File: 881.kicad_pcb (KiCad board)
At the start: 2 copper layers, 38 x 105 mm, 79 parts, among them J1 BD TRIG, J10 CY TRIG, J11 OH TRIG, J12 CH_TRIG, J13 ACCENT IN, J14 RUN/STOP, J15 RESET, J16 CLOCK OUT, J17 ACCENT OUT, J2 SD TRIG, J3 LT TRIG, J4 MT TRIG, J5 HT_TRIG, J6 RS TRIG, J7 CP_TRIG, J8 MA_TRIG, J9 CB TRIG, P1 CONN_02X03, P2 CONN_02X10, SW1 SPDT, U1 CD4048B, U2 CD4048B, X1 SYNC24 OUT, X2 MIDI OUT

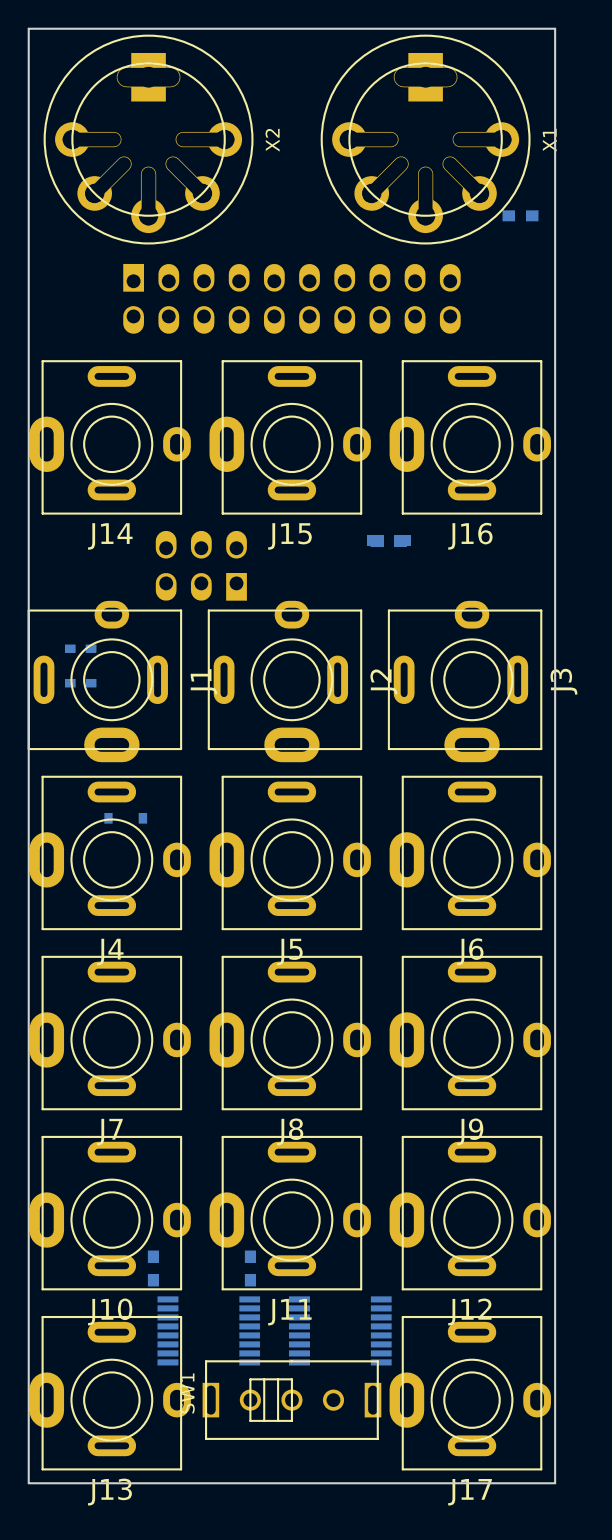
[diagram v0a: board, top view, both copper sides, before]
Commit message: placed and routed
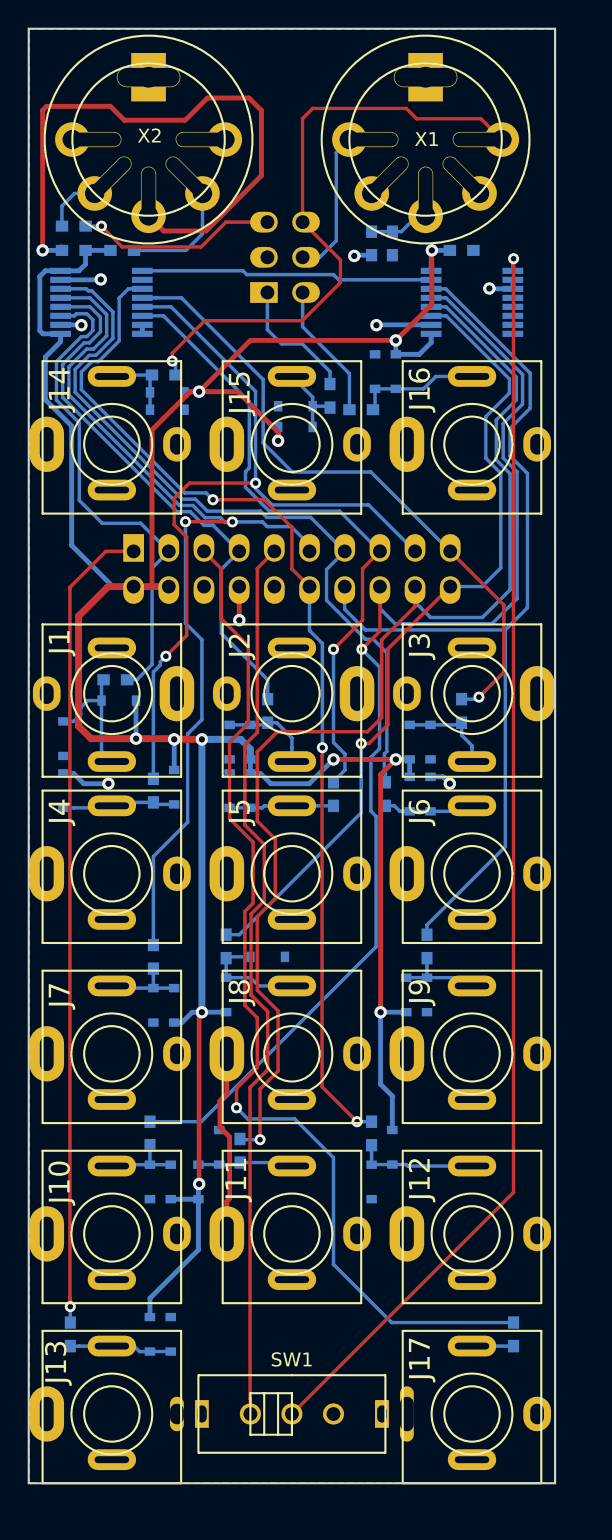
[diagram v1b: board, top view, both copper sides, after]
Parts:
- SW1: footprint MyModules:SS-12F45-1P2T-SLIDE -> MyModules:SS-12F108-1P2T-SLIDE
- moved C3 75.1 mm to (142.8, 71.0), turned to 0 degrees
- moved U2 74.9 mm to (143.5, 74.8)
- moved U1 74.7 mm to (116.8, 74.8)
- moved C2 73.7 mm to (114.8, 71.0), turned to 180 degrees
- moved R16 61.7 mm to (114.5, 149.2), turned to 90 degrees
- moved D25 59.8 mm to (120.2, 149.2), turned to 90 degrees
- moved D26 59.4 mm to (121.8, 149.2), turned to 270 degrees
- moved R20 58.0 mm to (146.5, 149.2), turned to 90 degrees
- moved D20 49.4 mm to (120.2, 138.2), turned to 90 degrees
- moved D19 48.9 mm to (121.8, 138.2), turned to 270 degrees
- moved D21 48.3 mm to (123.8, 138.2), turned to 270 degrees
- moved D24 46.3 mm to (136.2, 138.2), turned to 90 degrees
- moved R12 46.1 mm to (120.2, 134.8), turned to 90 degrees
- moved D22 45.5 mm to (125.2, 135.8), turned to 270 degrees
- moved R13 45.3 mm to (126.8, 136.0), turned to 90 degrees
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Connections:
- U1 pad 11: /RS_TRIG -> /BD_TRIG
- U1 pad 12: /CP_TRIG -> /SD_TRIG
- U1 pad 13: /SD_TRIG -> /CP_TRIG
- U1 pad 14: /BD_TRIG -> /RS_TRIG
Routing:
- net +5V: track 0.00 -> 218.0 mm, vias 0 -> 12
- net Net-(SW1-Pad2): track 0.00 -> 90.9 mm, vias 0 -> 1
- net /CY_TRIG: track 0.00 -> 87.8 mm, vias 0 -> 1
- net /OH_TRIG: track 0.00 -> 86.1 mm, vias 0 -> 1
- net GND: track 0.00 -> 76.8 mm, vias 0 -> 9
- net COMMON_TRIG: track 0.00 -> 75.4 mm, vias 0 -> 1
- net /CH_TRIG: track 0.00 -> 75.2 mm, vias 0 -> 3
- net /CP_TRIG: track 0.00 -> 69.3 mm, vias 0 -> 2
- net /CB_TRIG: track 0.00 -> 68.2 mm
- net /TRIG: track 0.00 -> 65.2 mm
- net /MA_TRIG: track 0.00 -> 59.3 mm, vias 0 -> 1
- net /MT_TRIG: track 0.00 -> 59.1 mm, vias 0 -> 2
- net /ACCENT: track 0.00 -> 58.8 mm, vias 0 -> 1
- net /RS_TRIG: track 0.00 -> 55.3 mm
- net /LT_TRIG: track 0.00 -> 47.2 mm, vias 0 -> 1
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- added copper zone on B.Cu, net GND
- added copper zone on F.Cu, net GND
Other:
- net class Default: via_dia 0.6 -> 0.8
- net class POWER added: clearance 0.25, trace_width 0.35, via_dia 0.9, via_drill 0.45
